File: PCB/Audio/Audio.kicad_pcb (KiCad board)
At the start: 2 copper layers, 70 x 70 mm, 36 parts, among them J1 JST-PH-SM4-TB, J3 TC2030-USB-NL-DS, J4 TF_PUSH, J5 USB-C-Socket-H, Q2 CJ2301, SW1 SW_Push, U1 L, U2 R, U3 TP4054, U4 ME6211C33M5G-N, U6 ESP32-S3-MINI-1

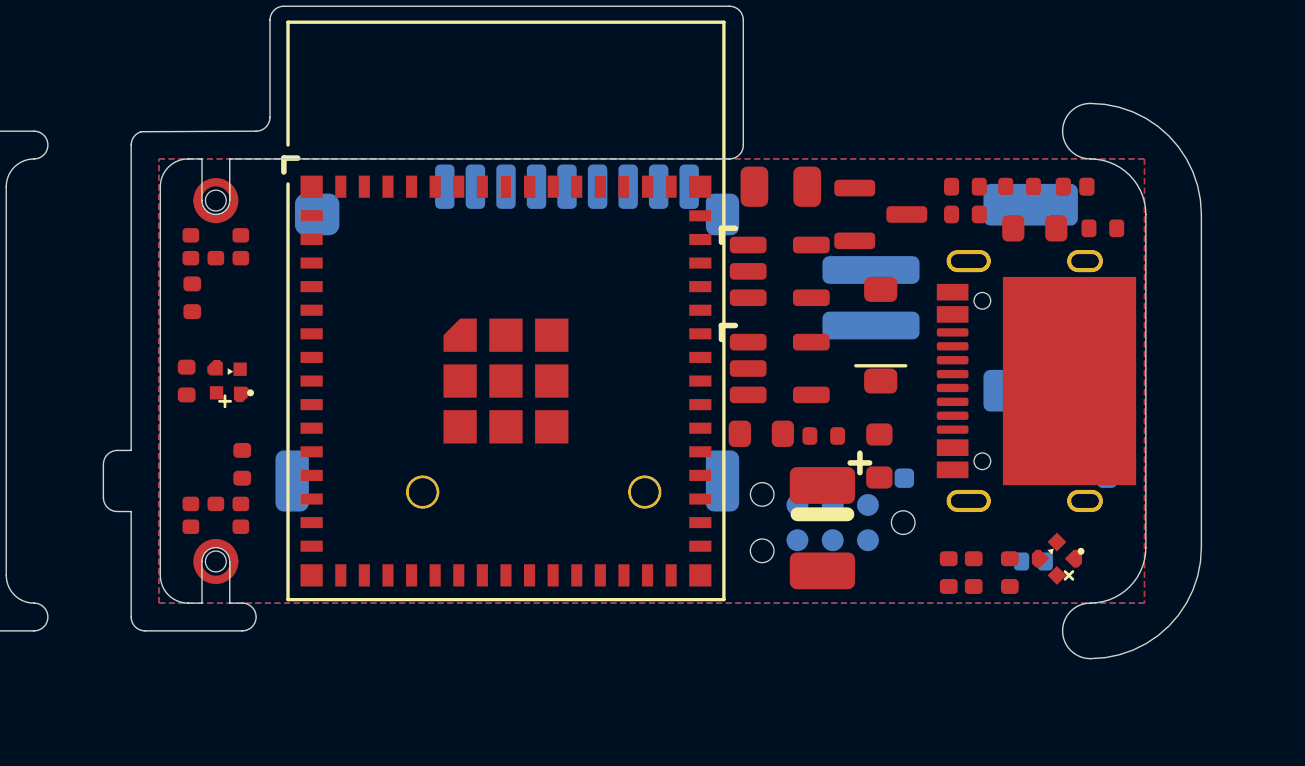
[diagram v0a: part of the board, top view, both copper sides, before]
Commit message: Initial tracking
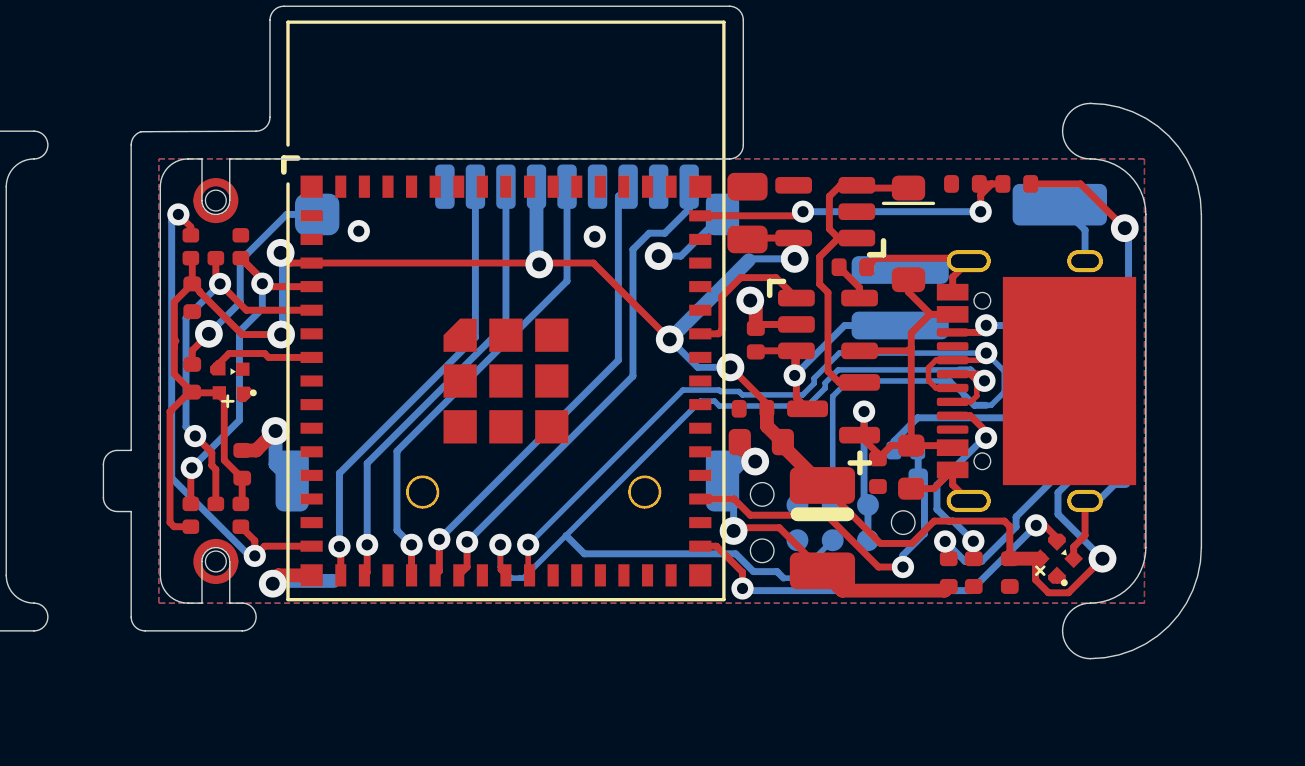
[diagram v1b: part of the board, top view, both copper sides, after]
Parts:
- removed C7: 10uF 35V, RevK:C_0603
- moved D2 12.8 mm to (109.0, 98.5), turned to -90 degrees
- moved R8 11.5 mm to (113.4, 103.3), turned to -90 degrees
- moved R1 9.11 mm to (112.5, 95.9), turned to 180 degrees
- moved Q2 7.20 mm to (111.8, 101.0), turned to 180 degrees
- moved D4 6.10 mm to (114.4, 102.5)
- moved D3 3.78 mm to (114.5, 94.7), turned to -90 degrees
- moved C2 2.73 mm to (108.9, 101.0), turned to 180 degrees
- moved U4 2.70 mm to (111.5, 93.9), turned to 180 degrees
- moved U3 2.35 mm to (111.6, 98.0)
- moved R2 1.85 mm to (118.4, 92.9)
- moved C16 1.55 mm to (108.7, 93.8), turned to 90 degrees
- moved C5 1.22 mm to (114.6, 103.1)
- moved C9 1.10 mm to (116.5, 92.9)
- moved J1 1.05 mm to (117.0, 97.0)
- moved SW1 0.50 mm to (118.5, 103.5)
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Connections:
- C16 pad 1: +3.3V -> +3V3
- C5 pad 1: DC -> VBUS
- J3 pad 1: DC -> VBUS
- J3 pad 2: DC -> VBUS
- J4 pad 4: SPWR -> +3V3
- J5 pad A4: DC -> VBUS
- J5 pad A9: DC -> VBUS
- J5 pad B4: DC -> VBUS
- J5 pad B9: DC -> VBUS
- U4 pad 5: +3.3V -> +3V3
- U6 pad 10: PUSH -> unconnected-(U6-GPIO6-Pad10)
- U6 pad 12: ADC -> unconnected-(U6-GPIO8-Pad12)
- U6 pad 15: unconnected-(U6-GPIO11-Pad15) -> SCK
- U6 pad 16: unconnected-(U6-GPIO12-Pad16) -> SDSS
- U6 pad 17: unconnected-(U6-GPIO13-Pad17) -> SDMOSI
- U6 pad 19: unconnected-(U6-GPIO15-Pad19) -> SDSCK
- U6 pad 20: unconnected-(U6-GPIO16-Pad20) -> SDMISO
- U6 pad 21: unconnected-(U6-GPIO17-Pad21) -> SDCD
- U6 pad 33: unconnected-(U6-GPIO37-Pad33) -> BUTTON
- U6 pad 36: SD -> unconnected-(U6-GPIO40-Pad36)
- U6 pad 37: WS -> unconnected-(U6-GPIO41-Pad37)
- U6 pad 38: SCK -> unconnected-(U6-GPIO42-Pad38)
- U6 pad 4: unconnected-(U6-GPIO0-Pad4) -> WS
- U6 pad 40: unconnected-(U6-GPIO44-Pad40) -> CHARGING
- U6 pad 5: unconnected-(U6-GPIO1-Pad5) -> SD
- U6 pad 7: unconnected-(U6-GPIO3-Pad7) -> BLINK2
- U6 pad 8: LED -> unconnected-(U6-GPIO4-Pad8)
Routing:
- net +3V3: track 0.00 -> 94.8 mm, vias 0 -> 8
- net GND: track 0.00 -> 55.6 mm, vias 0 -> 9
- net D-: track 0.00 -> 37.7 mm, vias 0 -> 2
- net D+: track 0.00 -> 37.0 mm, vias 0 -> 2
- net VBUS: track 0.00 -> 19.8 mm, vias 0 -> 1
- net SCK: track 0.00 -> 18.1 mm, vias 0 -> 2
- net Net-(J5-CC2): track 0.00 -> 17.9 mm, vias 0 -> 2
- net SDCD: track 0.00 -> 17.8 mm, vias 0 -> 1
- net SDMISO: track 0.00 -> 16.9 mm, vias 0 -> 1
- net SDSCK: track 0.00 -> 16.8 mm, vias 0 -> 1
- net SDMOSI: track 0.00 -> 16.1 mm, vias 0 -> 1
- net SDSS: track 0.00 -> 16.0 mm, vias 0 -> 1
- net BLINK: track 0.00 -> 15.0 mm, vias 0 -> 2
- net SD: track 0.00 -> 13.6 mm, vias 0 -> 2
- net WS: track 0.00 -> 13.2 mm, vias 0 -> 2
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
